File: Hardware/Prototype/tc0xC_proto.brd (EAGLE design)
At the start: 101.6 x 98.8 mm, 96 parts, among them IC1 AP2112M-3.3TRG1, Q1 2.5A/30V, Q2 MBT3904DW1T1, Q3 600mA/40V, Q4 MBT3904DW1T1, U2 ESP3212, U4 FT231XS, U5 W25Q32FVSS, Y1 26MHz, Y2 32.768kHz

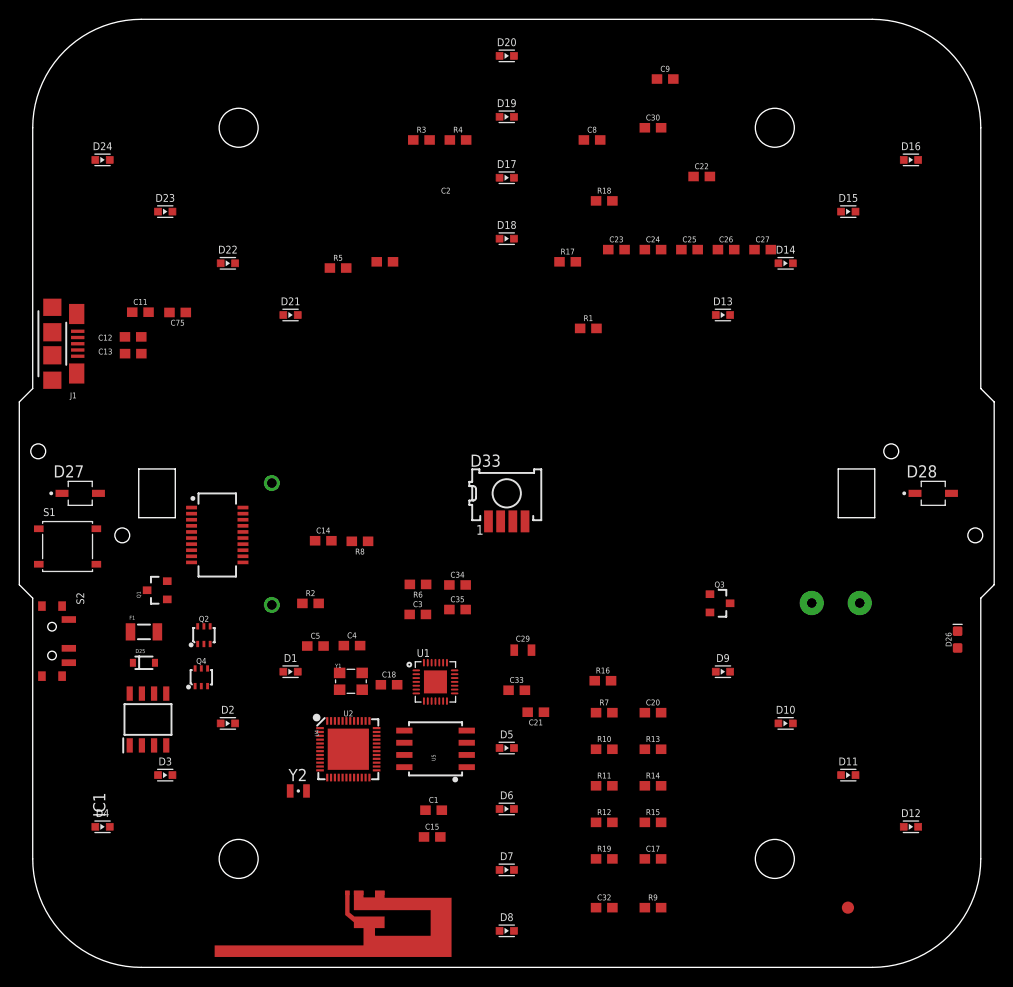
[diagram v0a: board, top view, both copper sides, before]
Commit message: cleaned ripped up prototype
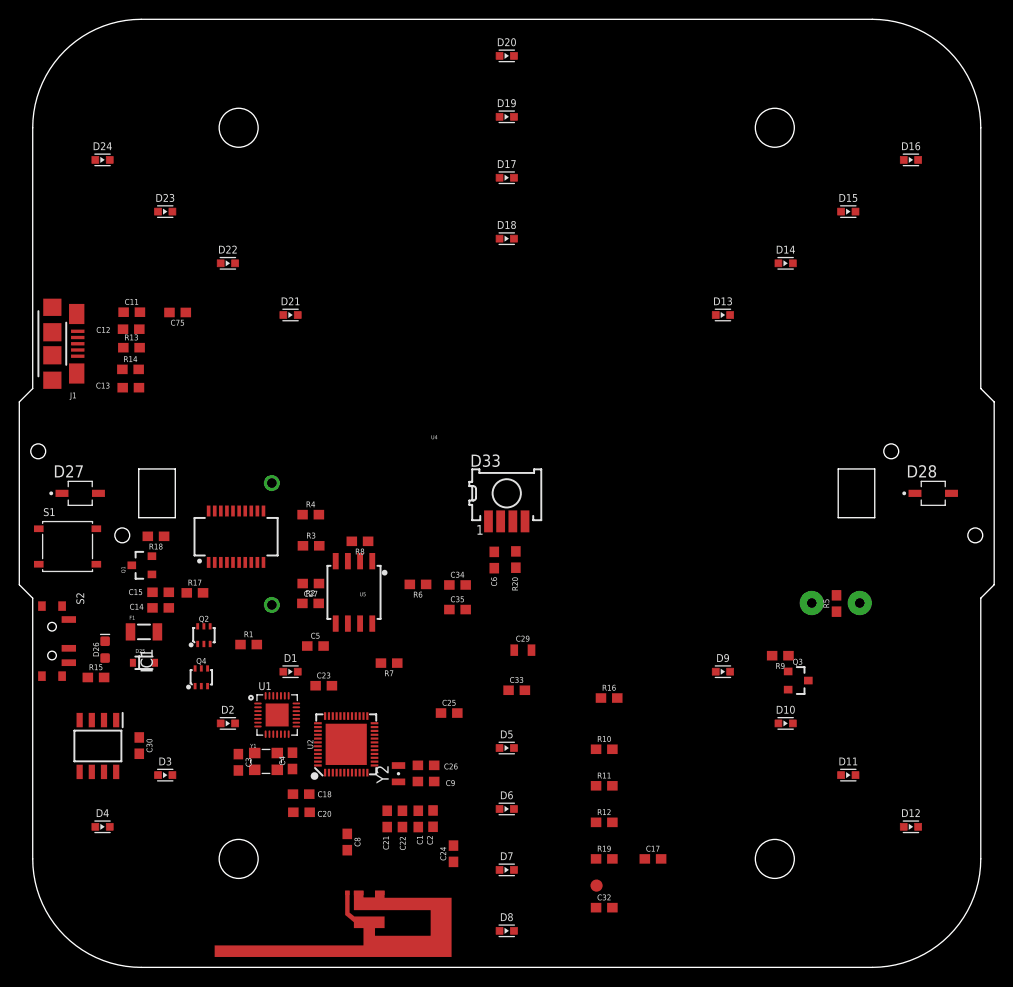
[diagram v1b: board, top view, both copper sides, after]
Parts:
- added C6: 4.7uF, SparkFun-Capacitors:0603
- added R20: 100, SparkFun-Resistors:0603
- moved D26 88.9 mm to (8.94, 34.5)
- moved C30 83.7 mm to (12.5, 24.5), turned to 270 degrees
- moved C8 77.5 mm to (34.2, 14.5), turned to 270 degrees
- moved C9 77.3 mm to (42.4, 20.8), turned to 180 degrees
- moved C22 73.9 mm to (39.9, 16.9), turned to 90 degrees
- moved R14 69.6 mm to (11.6, 63.7)
- moved R13 68.6 mm to (11.7, 66.0)
- moved C24 66.3 mm to (45.2, 13.2), turned to 90 degrees
- moved R5 62.6 mm to (85.2, 39.3), turned to 90 degrees
- moved C26 62.2 mm to (42.4, 22.4), turned to 180 degrees
- moved R15 60.0 mm to (7.99, 31.6)
- moved C27 58.6 mm to (30.4, 41.4), turned to 180 degrees
- moved R18 58.4 mm to (14.2, 46.3), turned to 180 degrees
- moved C2 58.2 mm to (43.1, 16.9), turned to 90 degrees
- moved C23 54.7 mm to (31.7, 30.8)
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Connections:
- removed net VS: D33.3
- net 3.3V: now also C6.1, D33.3, R20.1, R20.2
- net ACC_INT: now also D33.4
- net GND: now also C6.2

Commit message: matrixed LEDs
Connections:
- new net N$21: D13.P$1, D14.P$1, D15.P$1, D16.P$1
- new net N$22: D17.P$1, D18.P$1, D19.P$1, D20.P$1
- new net N$6: D21.P$1, D22.P$1, D23.P$1, D24.P$1
- net CA1: now also D1.P$2, D13.P$2, D17.P$2, D2.P$1, D21.P$2, D3.P$1, D4.P$1, D5.P$2, D9.P$2
- net CA2: now also D1.P$1, D10.P$2, D14.P$2, D18.P$2, D2.P$2, D22.P$2, D6.P$2, D7.P$1, D8.P$1
- net CA3: now also D11.P$2, D12.P$1, D15.P$2, D19.P$2, D23.P$2, D3.P$2, D5.P$1, D6.P$1, D7.P$2
- net CA4: now also D10.P$1, D11.P$1, D12.P$2, D16.P$2, D20.P$2, D24.P$2, D4.P$2, D8.P$2, D9.P$1
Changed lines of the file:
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@@
 <signal name="CA1">
 <contactref element="U1" pad="21"/>
+<contactref element="D21" pad="P$2"/>
+<contactref element="D1" pad="P$2"/>
+<contactref element="D5" pad="P$2"/>
+<contactref element="D9" pad="P$2"/>
+<contactref element="D13" pad="P$2"/>
+<contactref element="D17" pad="P$2"/>
+<contactref element="D2" pad="P$1"/>
+<contactref element="D4" pad="P$1"/>
+<contactref element="D3" pad="P$1"/>
+<wire x1="51.55" y1="83.693" x2="74.082340625" y2="69.38771875" width="0" layer="19" extent="1-1"/>
+<wire x1="29.017659375" y1="69.38771875" x2="51.55" y2="83.693" width="0" layer="19" extent="1-1"/>
+<wire x1="74.082340625" y1="32.21228125" x2="74.082340625" y2="69.38771875" width="0" layer="19" extent="1-1"/>
+<wire x1="51.55" y1="24.257" x2="74.082340625" y2="32.21228125" width="0" layer="19" extent="1-1"/>
+<wire x1="28.87" y1="28.9" x2="51.55" y2="24.257" width="0" layer="19" extent="1-1"/>
+<wire x1="29.017659375" y1="32.21228125" x2="28.87" y2="28.9" width="0" layer="19" extent="1-1"/>
+<wire x1="20.98731875" y1="26.8224" x2="28.87" y2="28.9" width="0" layer="19" extent="1-1"/>
+<wire x1="14.45698125" y1="21.435059375" x2="20.98731875" y2="26.8224" width="0" layer="19" extent="1-1"/>
+<wire x1="7.9241" y1="16.04771875" x2="14.45698125" y2="21.435059375" width="0" layer="19" extent="1-1"/>
 </signal>
 <signal name="CA2">
 <contactref element="U1" pad="22"/>
+<contactref element="D22" pad="P$2"/>
+<contactref element="D2" pad="P$2"/>
+<contactref element="D6" pad="P$2"/>
+<contactref element="D10" pad="P$2"/>
+<contactref element="D14" pad="P$2"/>
+<contactref element="D18" pad="P$2"/>
+<contactref element="D1" pad="P$1"/>
+<contactref element="D7" pad="P$1"/>
+<contactref element="D8" pad="P$1"/>
+<wire x1="51.55" y1="77.343" x2="80.615221875" y2="74.775059375" width="0" layer="19" extent="1-1"/>
+<wire x1="22.48731875" y1="74.775059375" x2="51.55" y2="77.343" width="0" layer="19" extent="1-1"/>
+<wire x1="27.517659375" y1="32.21228125" x2="22.48731875" y2="74.775059375" width="0" layer="19" extent="1-1"/>
+<wire x1="28.07" y1="29.7" x2="27.517659375" y2="32.21228125" width="0" layer="19" extent="1-1"/>
+<wire x1="22.48731875" y1="26.8224" x2="28.07" y2="29.7" width="0" layer="19" extent="1-1"/>
+<wire x1="51.55" y1="17.907" x2="28.07" y2="29.7" width="0" layer="19" extent="1-1"/>
+<wire x1="50.05" y1="11.557" x2="51.55" y2="17.907" width="0" layer="19" extent="1-1"/>
+<wire x1="50.05" y1="5.207" x2="50.05" y2="11.557" width="0" layer="19" extent="1-1"/>
+<wire x1="80.615221875" y1="26.8224" x2="51.55" y2="17.907" width="0" layer="19" extent="1-1"/>
 </signal>
 <signal name="CA3">
 <contactref element="U1" pad="23"/>
+<contactref element="D5" pad="P$1"/>
+<contactref element="D6" pad="P$1"/>
+<contactref element="D23" pad="P$2"/>
+<contactref element="D3" pad="P$2"/>
+<contactref element="D7" pad="P$2"/>
+<contactref element="D11" pad="P$2"/>
+<contactref element="D15" pad="P$2"/>
+<contactref element="D19" pad="P$2"/>
+<contactref element="D12" pad="P$1"/>
+<wire x1="51.55" y1="90.043" x2="87.145559375" y2="80.1624" width="0" layer="19" extent="1-1"/>
+<wire x1="15.95698125" y1="80.1624" x2="51.55" y2="90.043" width="0" layer="19" extent="1-1"/>
+<wire x1="27.67" y1="29.7" x2="15.95698125" y2="80.1624" width="0" layer="19" extent="1-1"/>
+<wire x1="15.95698125" y1="21.435059375" x2="27.67" y2="29.7" width="0" layer="19" extent="1-1"/>
+<wire x1="50.05" y1="24.257" x2="27.67" y2="29.7" width="0" layer="19" extent="1-1"/>
+<wire x1="50.05" y1="17.907" x2="50.05" y2="24.257" width="0" layer="19" extent="1-1"/>
+<wire x1="51.55" y1="11.557" x2="50.05" y2="17.907" width="0" layer="19" extent="1-1"/>
+<wire x1="87.145559375" y1="21.435059375" x2="51.55" y2="11.557" width="0" layer="19" extent="1-1"/>
+<wire x1="92.1759" y1="16.04771875" x2="87.145559375" y2="21.435059375" width="0" layer="19" extent="1-1"/>
 </signal>
 <signal name="CA8">
@@
 <signal name="CA4">
 <contactref element="U1" pad="24"/>
+<contactref element="D9" pad="P$1"/>
+<contactref element="D10" pad="P$1"/>
+<contactref element="D11" pad="P$1"/>
+<contactref element="D24" pad="P$2"/>
+<contactref element="D16" pad="P$2"/>
+<contactref element="D20" pad="P$2"/>
+<contactref element="D12" pad="P$2"/>
+<contactref element="D8" pad="P$2"/>
+<contactref element="D4" pad="P$2"/>
+<wire x1="51.55" y1="96.393" x2="93.6759" y2="85.55228125" width="0" layer="19" extent="1-1"/>
+<wire x1="9.4241" y1="85.55228125" x2="51.55" y2="96.393" width="0" layer="19" extent="1-1"/>
+<wire x1="72.582340625" y1="32.21228125" x2="93.6759" y2="85.55228125" width="0" layer="19" extent="1-1"/>
+<wire x1="79.115221875" y1="26.8224" x2="72.582340625" y2="32.21228125" width="0" layer="19" extent="1-1"/>
+<wire x1="85.645559375" y1="21.435059375" x2="79.115221875" y2="26.8224" width="0" layer="19" extent="1-1"/>
+<wire x1="93.6759" y1="16.04771875" x2="85.645559375" y2="21.435059375" width="0" layer="19" extent="1-1"/>
+<wire x1="51.55" y1="5.207" x2="72.582340625" y2="32.21228125" width="0" layer="19" extent="1-1"/>
+<wire x1="27.27" y1="29.7" x2="51.55" y2="5.207" width="0" layer="19" extent="1-1"/>
+<wire x1="9.4241" y1="16.04771875" x2="27.27" y2="29.7" width="0" layer="19" extent="1-1"/>
 </signal>
 <signal name="CA5">
@@
 <contactref element="U1" pad="27"/>
 </signal>
+<signal name="N$6">
+<contactref element="D21" pad="P$1"/>
+<contactref element="D22" pad="P$1"/>
+<contactref element="D23" pad="P$1"/>
+<contactref element="D24" pad="P$1"/>
+<wire x1="20.98731875" y1="74.775059375" x2="27.517659375" y2="69.38771875" width="0" layer="19" extent="1-1"/>
+<wire x1="14.45698125" y1="80.1624" x2="20.98731875" y2="74.775059375" width="0" layer="19" extent="1-1"/>
+<wire x1="7.9241" y1="85.55228125" x2="14.45698125" y2="80.1624" width="0" layer="19" extent="1-1"/>
+</signal>
+<signal name="N$21">
+<contactref element="D13" pad="P$1"/>
+<contactref element="D14" pad="P$1"/>
+<contactref element="D15" pad="P$1"/>
+<contactref element="D16" pad="P$1"/>
+<wire x1="85.645559375" y1="80.1624" x2="92.1759" y2="85.55228125" width="0" layer="19" extent="1-1"/>
+<wire x1="79.115221875" y1="74.775059375" x2="85.645559375" y2="80.1624" width="0" layer="19" extent="1-1"/>
+<wire x1="72.582340625" y1="69.38771875" x2="79.115221875" y2="74.775059375" width="0" layer="19" extent="1-1"/>
+</signal>
+<signal name="N$22">
+<contactref element="D17" pad="P$1"/>
+<contactref element="D18" pad="P$1"/>
+<contactref element="D19" pad="P$1"/>
+<contactref element="D20" pad="P$1"/>
+<wire x1="50.05" y1="90.043" x2="50.05" y2="96.393" width="0" layer="19" extent="1-1"/>
+<wire x1="50.05" y1="83.693" x2="50.05" y2="90.043" width="0" layer="19" extent="1-1"/>
+<wire x1="50.05" y1="77.343" x2="50.05" y2="83.693" width="0" layer="19" extent="1-1"/>
+</signal>
 </signals>
